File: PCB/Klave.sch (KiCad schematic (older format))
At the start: 78 parts, among them J1 6P6C, J2 OLED, SW0 Reset, SW1 0:0, SW10 1:3, SW11 1:4, SW12 1:5, SW13 2:0, SW14 2:1, SW15 2:2, SW16 2:3, SW17 2:4, SW18 2:5, SW19 3:0, SW2 0:1, SW20 3:1, SW21 3:2, SW22 3:3, SW23 3:4, SW24 3:5, SW26 4:1, SW27 4:2, SW28 4:3, SW29 4:4, SW3 0:2, SW30 4:5, SW35 5:4, SW36 5:5, SW4 0:3, SW5 0:4, SW6 0:5, SW7 1:0, SW8 1:1, SW9 1:2, U1 ProMicro

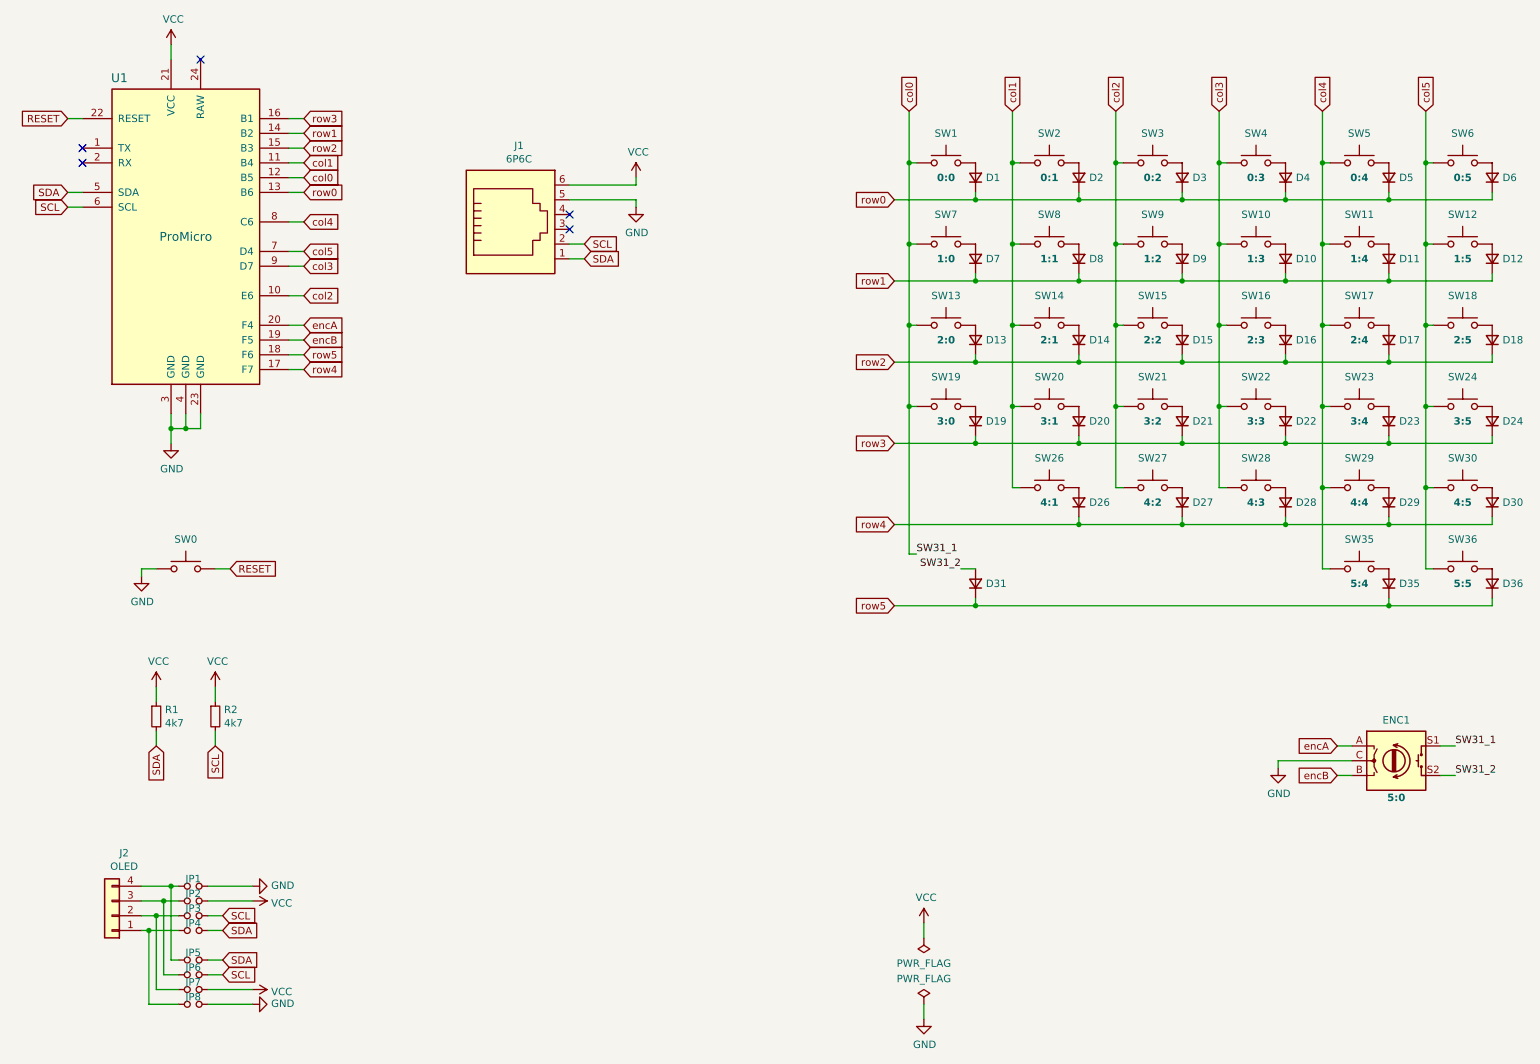
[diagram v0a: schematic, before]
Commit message: Apply schematic "best practices"
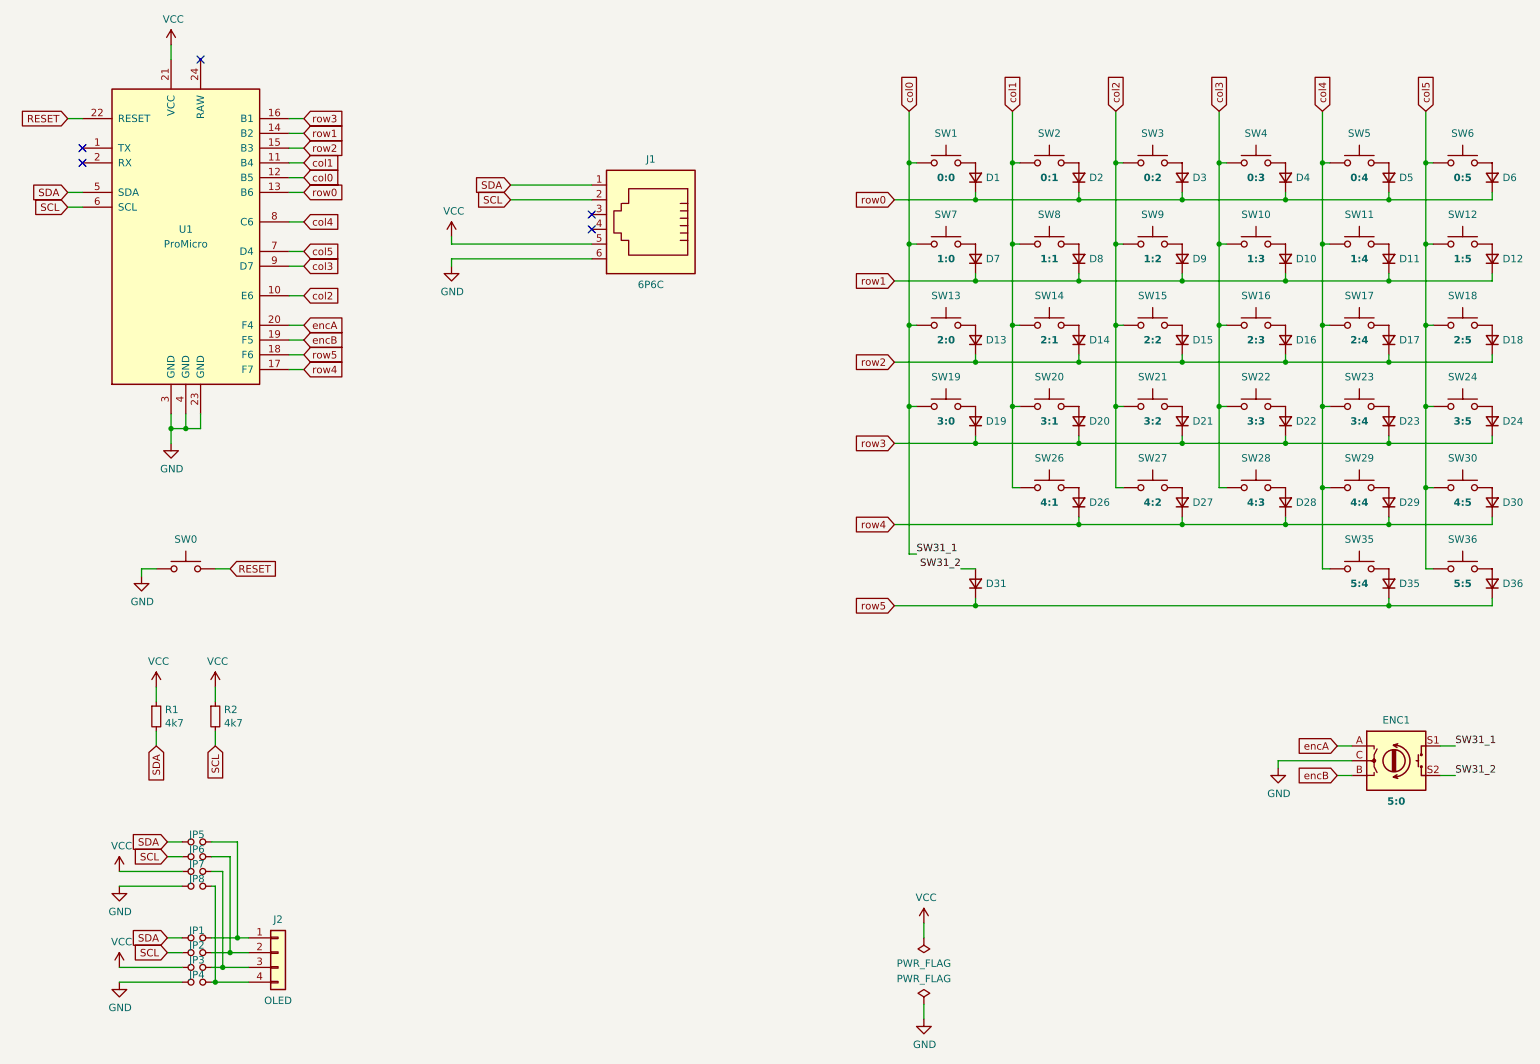
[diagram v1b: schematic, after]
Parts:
- renumbered JP4 to JP1, JP3 to JP2, JP2 to JP3, JP1 to JP4
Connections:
- net GND: now also J1.6; no longer J1.5
- net VCC: now also J1.5; no longer J1.6
- net at J2.1 (Pin_1), JP1.1: now also JP5.1; no longer JP8.1
- net at J2.2 (Pin_2), JP2.1: now also JP6.1; no longer JP7.1
- net at J2.3 (Pin_3), JP3.1: now also JP7.1; no longer JP6.1
- net at J2.4 (Pin_4), JP4.1: now also JP8.1; no longer JP5.1
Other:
- moved on the sheet: J1, J2, JP1, JP2, JP3, JP4, JP5, JP6, JP7, JP8
